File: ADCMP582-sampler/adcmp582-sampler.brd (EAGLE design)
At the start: 160 x 100 mm, 62 parts, among them IC12 MC79M05, IC13 MC78M05, IC2 MC100EPT21, IC3 SY89296U, IC6 AD711

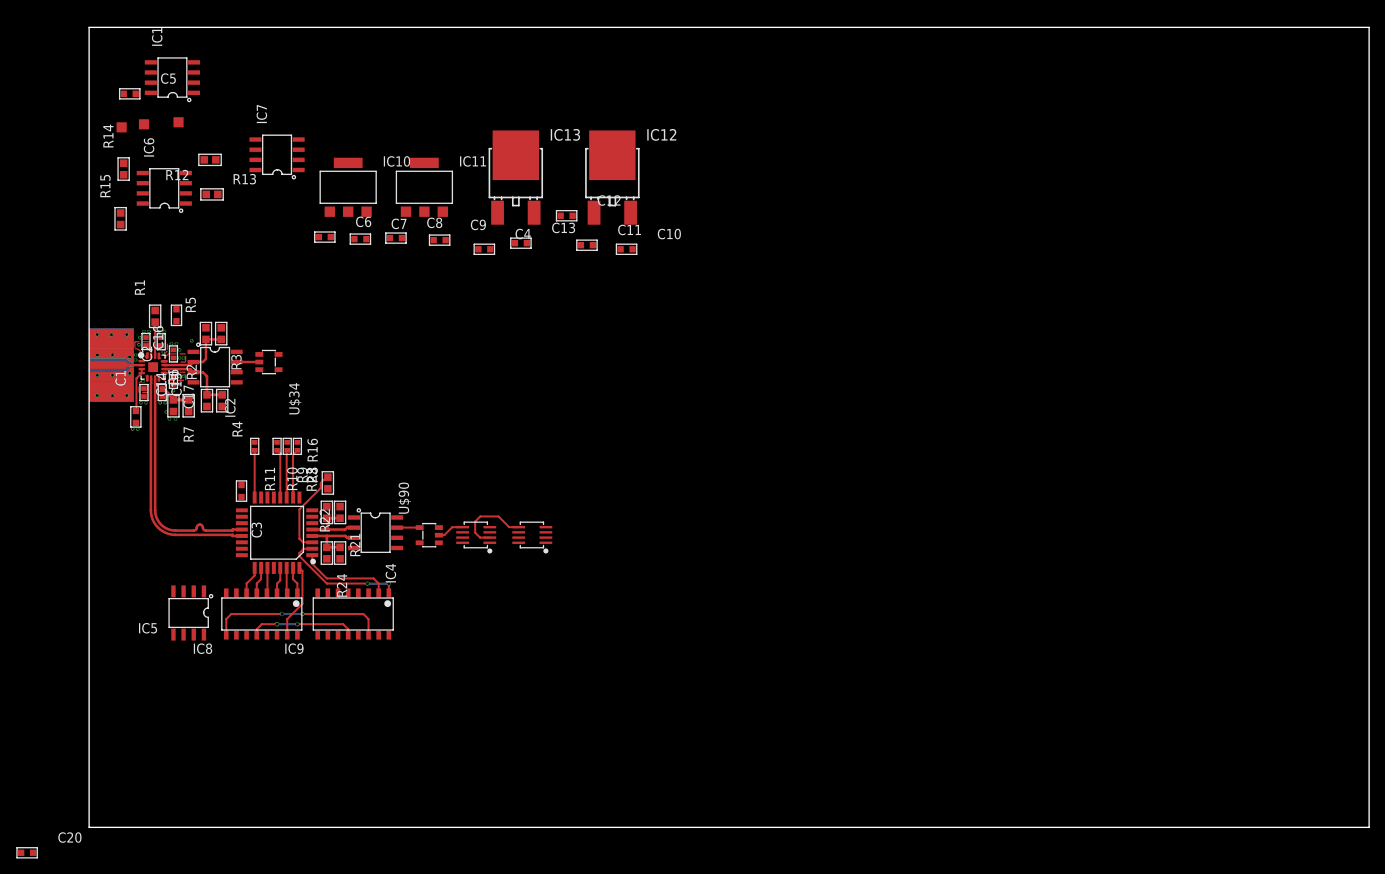
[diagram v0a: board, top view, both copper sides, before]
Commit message: checkpoint
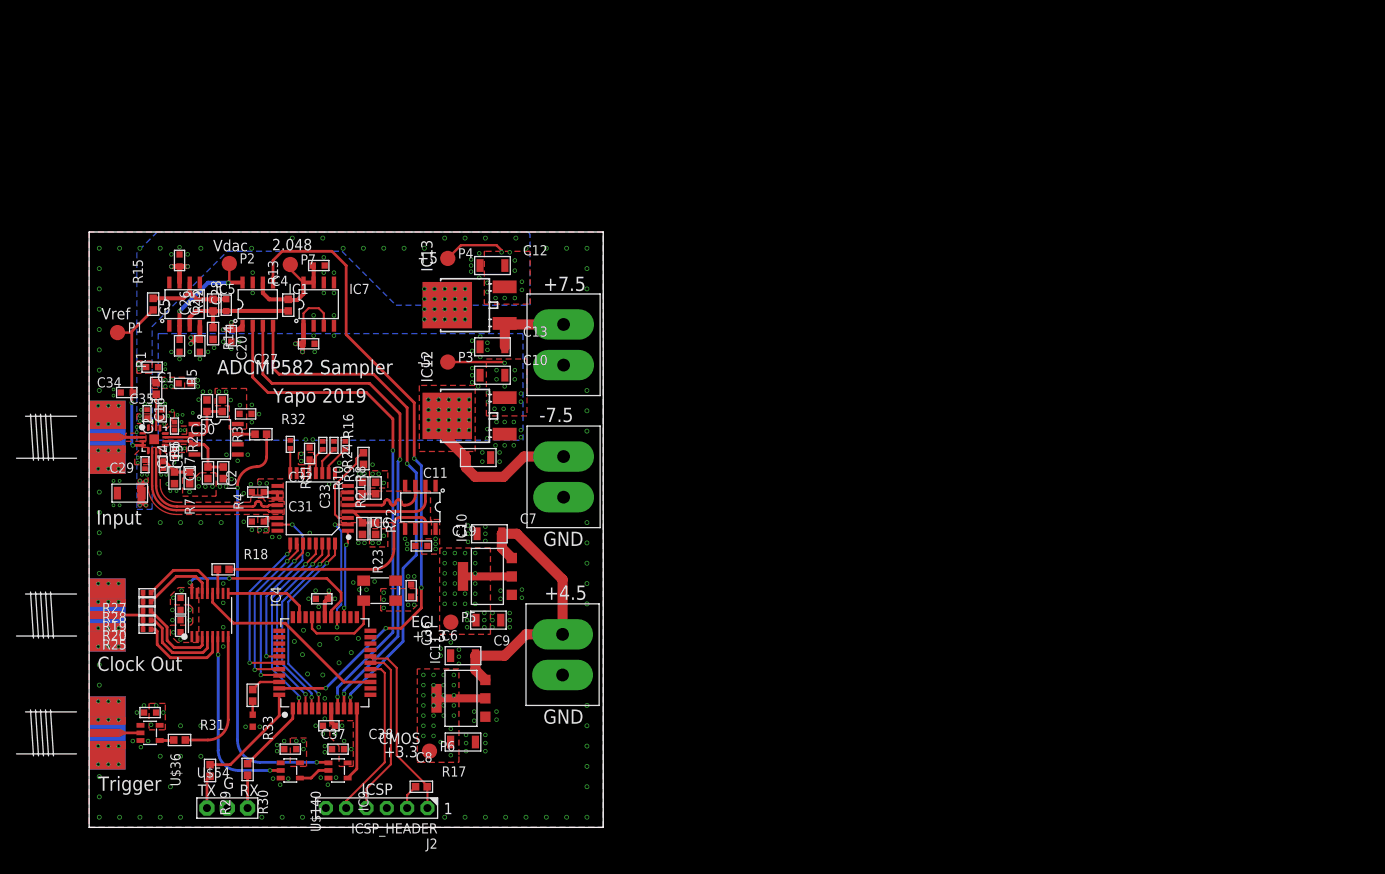
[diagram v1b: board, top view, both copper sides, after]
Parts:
- removed IC14, IC15: (no value), yapo:SSOP8
- removed U$34, U$90: 74LVC1G04, yapo:SOT23-5
- removed U$46, U$47, U$48: PAD50MIL, yapo:PAD_50MIL
- added C21, C22, C23, C24, C25, C26, C27, C28, C30, C31, C32, C33, C34, C35, C36, C37, C38: (no value), yapo:C0603
- added C29: (no value), yapo:1206
- added J2: ICSP_HEADER, yapo:HEADER_6PIN
- added J3, J4: (no value), sma_footprint_2l:SMA_EDGE_LAUNCH_4L_4020_TAPER_FIXED
- added J5, J6, J7: (no value), yapo:FCI_20020316_SCREW_TERM_2P
- added P1, P2, P3, P4, P5, P6, P7: ICSP_PAD, yapo:ICSP_PAD
- added R17, R18, R29, R30, R31, R32, R33: (no value), yapo:R0603
- added R19, R20, R25, R27, R28: (no value), yapo:0402
- added U$140: 74LVC1G04, yapo:SOT23-5
- added U$36: (no value), yapo:SOT23-5
- added U$54: HEADER_3PIN, yapo:HEADER_3PIN
- added U$88: LED_0603, yapo:LED_0603
- added X1: (no value), yapo:XTAL_3.2X5
- C10, C11, C12, C13, C6, C7, C8, C9: device yapo:C0603 -> yapo:1206
- IC4: device yapo:SOIC8 -> yapo:TQFP44
- IC6: value AD711 -> (none)
- IC8: device yapo:SOIC-16 -> yapo:TSSOP16
- IC9: device yapo:SOIC-16 -> yapo:SOT23-5
- J1: device yapo:SMA_EDGE_LAUNCH -> sma_footprint_2l:SMA_EDGE_LAUNCH_4L_4020_TAPER_FIXED
- moved C20 72.8 mm to (17.1, 65.3), turned to 270 degrees
- moved IC11 64.0 mm to (46.5, 16.1), turned to 90 degrees
- moved C8 63.5 mm to (46.7, 10.7), turned to 180 degrees
- moved C6 52.1 mm to (49.9, 25.9), turned to 180 degrees
- moved C9 52.0 mm to (46.7, 21.5)
- moved IC10 51.7 mm to (49.8, 31.4), turned to 90 degrees
- moved IC6 51.1 mm to (41.4, 40.0), turned to 180 degrees
- moved C19 42.0 mm to (41.5, 35.2), turned to 0 degrees
- moved C7 40.2 mm to (50.0, 36.7)
- moved IC5 38.6 mm to (11.9, 65.4), turned to 0 degrees
- moved C5 32.1 mm to (11.3, 60.2), turned to 90 degrees
- moved IC1 30.3 mm to (21.1, 65.4), turned to 0 degrees
- moved C11 29.8 mm to (48.6, 46.2), turned to 180 degrees
- moved IC12 28.7 mm to (51.9, 51.4), turned to 90 degrees
- moved C10 23.0 mm to (50.4, 56.5)
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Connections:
- net LE_P renamed LE_P1
- removed net N$28: C9.P$2, IC11.3
- removed net N$29: C6.P$2, IC10.2, IC10.4
- removed net N$30: C8.P$2, IC11.2, IC11.4
- removed net N$31: C11.P$2, IC12.4
- removed net N$32: C10.P$2, IC12.3
- removed net N$33: C13.P$2, IC13.1
- removed net N$34: C12.P$2, IC13.3
- removed net N$40: IC14.1, IC15.1
- removed net RCLK: IC8.12, IC9.12
- removed net SER: IC8.14
- removed net SRCLK: IC8.11, IC9.11
- removed net TUNE-!CS!: IC5.2
- removed net TUNE-SCK: IC5.3
- removed net TUNE-SDI: IC5.4
- new net !LDAC!: IC1.5, IC4.43
- new net !MCLR!: IC4.18, J2.1, R17.P$2
- new net CLK-SEL: IC4.27, IC8.16
- new net CLOCK-OUT: J4.CENTER@1, J4.P$3, R19.2, R20.2, R25.2, R27.2, R28.2
- new net COMP-CLK: IC4.14, IC8.12
- new net COMP-OUT: IC4.11, IC9.4
- new net COMP-REG-CLK: IC8.6, U$140.2
- new net ICSPCLK: IC4.16, J2.5
- new net ICSPDAT: IC4.17, J2.4
- new net INPUT: J1.CENTER@1, J1.P$3, U$1.2
- new net N$26: R33.P$2, U$88.A
- new net N$39: IC8.13, R27.1
- new net N$41: IC8.5, R25.1
- new net N$43: IC8.3, R19.1
- new net N$44: IC4.44, R29.P$1
- new net N$45: IC4.1, R30.P$1
- new net N$47: IC4.35
- new net N$48: IC4.36
- new net N$49: IC4.37
- new net N$52: IC3.17
- new net N$53: IC4.19
- new net N$54: IC4.20
- new net N$55: IC4.21
- new net N$56: IC4.22
- new net N$57: IC4.23
- new net N$58: IC4.24
- new net N$60: IC4.31
- new net RX: R30.P$2, U$54.3
- new net SAMPLE-CLOCK: IC4.32, IC8.9
- new net TRIGGER: J3.CENTER@1, J3.P$3, U$36.2
- new net TX: R29.P$2, U$54.1
- new net VCC2: C22.P$2, C23.P$2, C24.P$2, C36.P$2, C37.P$2, C38.P$2, C8.P$2, IC11.2, IC11.4, IC4.28, IC4.7, IC9.5, J2.2, P6.P$1, R17.P$1, U$140.5, U$36.5, X1.4
- new net VDAC: C5.P$2, IC1.8, IC5.2, P2.P$1
- new net VIN+5: C13.P$2, IC13.1, J6.P$1
- new net VIN-5: C11.P$2, IC12.4, J5.P$1
- new net VIN3.3: C7.P$2, C9.P$2, IC10.3, IC11.3, J7.P$1
- net +3.3V: now also C19.P$2, C21.P$2, C27.P$2, C28.P$2, C3.P$2, C30.P$2, C31.P$2, C32.P$2, C33.P$2, C6.P$2, IC10.2, IC10.4, IC6.8, IC8.1, IC8.15, IC8.2, P5.P$1; no longer IC14.6, IC14.7, IC14.8, IC15.6, IC15.7, IC15.8, IC4.8, IC5.1, IC5.6, IC8.10, IC8.16, IC9.10, IC9.16, U$34.5, U$90.5
- net +5V: now also C12.P$2, C25.P$2, C29.P$2, C34.P$2, IC13.3, IC5.7, P4.P$1; no longer IC6.7
- net -5V: now also C10.P$2, C26.P$2, C35.P$2, IC12.3, IC5.4, P3.P$1; no longer C19.P$2, IC6.4, U$48.P$1
- net D0: now also IC4.38; no longer IC8.7
- net D1: now also IC4.39; no longer IC8.6
- net D2: now also IC4.40; no longer IC8.5
- net D3: now also IC4.41; no longer IC8.4
- net D4: now also IC4.2; no longer IC8.3
- net D5: now also IC4.3; no longer IC8.2
- net D6: now also IC4.4; no longer IC8.1
- net D7: now also IC4.5; no longer IC8.15
- net D8: now also IC4.25; no longer IC9.2
- net D9: now also IC4.26; no longer IC9.1
- net GND: now also C21.P$1, C22.P$1, C23.P$1, C24.P$1, C25.P$1, C26.P$1, C27.P$1, C28.P$1, C29.P$1, C30.P$1, C31.P$1, C32.P$1, C33.P$1, C34.P$1, C35.P$1, C36.P$1, C37.P$1, C38.P$1, IC4.29, IC4.6, IC6.5, IC8.10, IC8.7, IC9.3, J1.BOTTOM_GND, J1.P$1, J1.P$2, J2.3, J3.BOTTOM_GND, J3.GND@1, J3.GND@14, J3.GND@15, J3.GND@16, J3.GND@17, J3.GND@2, J3.GND@3, J3.GND@4, J3.GND@5, J3.GND@6, J3.GND@7, J3.GND@8, J3.GND_PAD1, J3.GND_PAD2, J3.P$1, J3.P$2, J4.BOTTOM_GND, J4.GND@1, J4.GND@14, J4.GND@15, J4.GND@16, J4.GND@17, J4.GND@2, J4.GND@3, J4.GND@4, J4.GND@5, J4.GND@6, J4.GND@7, J4.GND@8, J4.GND_PAD1, J4.GND_PAD2, J4.P$1, J4.P$2, J5.P$2, J6.P$2, J7.P$2, U$140.3, U$36.3, U$54.2, U$88.C, X1.2; no longer IC1.5, IC14.4, IC15.4, IC4.5, IC5.5, IC5.7, IC8.13, IC8.8, IC9.13, IC9.8, J1.BOTTOM_PAD, U$34.3, U$90.3
- net N$1: now also R31.P$1, U$36.4; no longer J1.CENTER@1, J1.CENTER@2, U$1.2
- net N$16: now also IC3.4, IC6.2; no longer IC3.5, IC4.2
- net N$17: now also IC2.7, R32.P$1; no longer IC3.4, IC4.3, R22.P$2, R24.P$1
- net N$18: now also IC8.11, R18.P$1; no longer C3.P$2, IC3.17, IC5.8
- net N$19: now also IC9.2, U$140.4; no longer IC2.7, U$34.2
- net N$20: now also IC5.3; no longer IC6.2
- net N$21: now also IC5.6; no longer IC6.6
- net N$22: now also IC3.5, R22.P$2, R24.P$1; no longer C5.P$2, IC1.8
- net N$23: now also IC8.8, R31.P$2; no longer IC6.1, U$47.P$1
- net N$24: now also IC4.30, X1.3; no longer IC6.5, U$46.P$1
- net N$25: now also IC4.42, R33.P$1; no longer IC8.9, IC9.14
- net N$27: now also IC9.1, R32.P$2; no longer C7.P$2, IC10.3
- net N$36: now also IC6.7, R18.P$2; no longer IC4.7, U$90.4
- net N$38: now also IC8.14, R28.1; no longer IC14.5, IC15.2
- net N$42: now also IC8.4, R20.1; no longer IC15.5, U$90.2
- net V2.048: now also P7.P$1
- net VREF: now also P1.P$1
- net VREF-!CS!: now also IC4.8
- net VREF-SCK: now also IC4.9
- net VREF-SDI: now also IC4.10
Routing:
- net !LDAC!: track 0.00 -> 81.7 mm, vias 0 -> 4
- net VREF-SDI: track 0.00 -> 65.6 mm, vias 0 -> 2
- net VREF-!CS!: track 0.00 -> 65.2 mm, vias 0 -> 2
- net VREF-SCK: track 0.00 -> 65.0 mm, vias 0 -> 2
- net N$27: track 0.00 -> 52.3 mm, vias 0 -> 2
- net VIN3.3: track 0.00 -> 35.9 mm
- net N$36: track 2.81 -> 30.2 mm
- net +3.3V: track 0.00 -> 26.3 mm, vias 4 -> 63
- net COMP-CLK: track 0.00 -> 25.0 mm
- net CLK-SEL: track 0.00 -> 24.9 mm, vias 0 -> 2
- net COMP-REG-CLK: track 0.00 -> 23.1 mm, vias 0 -> 2
- net !MCLR!: track 0.00 -> 23.0 mm
- net D0: track 0.00 -> 22.4 mm, vias 0 -> 2
- net ICSPDAT: track 0.00 -> 21.5 mm
- net D5: track 3.15 -> 24.4 mm, vias 0 -> 2
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- added copper zone on layer 15, net +3.3V
- added copper zone on layer 16, net +5V
- added copper zone on layer 16, net -5V
- added copper zone on layer 1, net GND
- added copper zone on layer 16, net GND
- added copper zone on layer 2, net GND
- added copper zone on layer 1, net VCC2
- added copper zone on layer 15, net VCC2
- added copper zone on layer 1, net VIN-5
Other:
- board size 160 x 100 mm -> 64.3 x 74.4 mm
- board text added: "+3.3"
- board text added: "+4.5"
- board text added: "+5"
- board text added: "+7.5"
- board text added: "-5"
- board text added: "-7.5"
- board text added: "1"
- board text added: "2.048"
- board text added: "ADCMP582 Sampler"
- board text added: "CMOS"
- board text added: "Clock Out"
- board text added: "ECL"
- board text added: "G"
- board text added: "GND"
- board text added: "ICSP"
- board text added: "Input"
- board text added: "RX"
- board text added: "TX"
- board text added: "Trigger"
- board text added: "Vdac"
- board text added: "Vref"
- board text added: "Yapo 2019"

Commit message: checkpoint
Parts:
- R12: value (none) -> 20k
- R13, R14: value (none) -> 10k
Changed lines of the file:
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@@
 <attribute name="VALUE" x="23.876" y="45.339" size="1.27" layer="27" rot="R270"/>
 </element>
-<element name="R12" library="yapo" package="R0603" value="" x="15.494" y="61.722" smashed="yes" rot="R90">
+<element name="R12" library="yapo" package="R0603" value="20k" x="15.494" y="61.722" smashed="yes" rot="R90">
 <attribute name="NAME" x="14.224" y="64.262" size="1.27" layer="25" rot="R90"/>
 <attribute name="VALUE" x="16.764" y="64.262" size="1.27" layer="27" rot="R90"/>
 </element>
-<element name="R13" library="yapo" package="R0603" value="" x="24.892" y="65.278" smashed="yes" rot="R90">
+<element name="R13" library="yapo" package="R0603" value="10k" x="24.892" y="65.278" smashed="yes" rot="R90">
 <attribute name="NAME" x="23.622" y="67.818" size="1.27" layer="25" rot="R90"/>
 <attribute name="VALUE" x="26.162" y="67.818" size="1.27" layer="27" rot="R90"/>
 </element>
-<element name="R14" library="yapo" package="R0603" value="" x="15.494" y="65.278" smashed="yes" rot="R270">
+<element name="R14" library="yapo" package="R0603" value="10k" x="15.494" y="65.278" smashed="yes" rot="R270">
 <attribute name="NAME" x="16.764" y="62.738" size="1.27" layer="25" rot="R270"/>
 <attribute name="VALUE" x="14.224" y="62.738" size="1.27" layer="27" rot="R270"/>
@@
 <contactref element="U$140" pad="2"/>
 <via x="16.129" y="21.59" extent="1-16" drill="0.35"/>
-<wire x1="16.129" y1="21.59" x2="16.129" y2="9.652" width="0.34925" layer="16"/>
+<wire x1="16.129" y1="9.652" x2="16.129" y2="21.59" width="0.34925" layer="16"/>
 <wire x1="16.129" y1="9.652" x2="18.669" y2="7.112" width="0.34925" layer="16" curve="90"/>
 <wire x1="18.669" y1="7.112" x2="22.606" y2="7.112" width="0.34925" layer="16"/>

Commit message: checkpoint
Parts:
- C1, C20, C4, C5, R15: value (none) -> 0
- IC1: value (none) -> MCP4921
- IC10, IC11: value (none) -> AZ1117E
- IC4: value (none) -> PIC16F15376
- IC5: value (none) -> ADA4000
- IC6: value (none) -> MC100LVELT20
- IC7: value (none) -> MCP1501
- IC8: value (none) -> SI53360
- IC9: value (none) -> 74LVC1G79
- U$36: value (none) -> 74LVC1G17
- X1: value (none) -> XTAL-3.2X5-8MHz
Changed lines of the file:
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@@
 </autorouter>
 <elements>
-<element name="C1" library="yapo" package="C0603" value="" x="4.699" y="54.356" smashed="yes">
+<element name="C1" library="yapo" package="C0603" value="0" x="4.699" y="54.356" smashed="yes">
 <attribute name="NAME" x="8.509" y="55.626" size="1.27" layer="25"/>
 <attribute name="VALUE" x="8.509" y="53.086" size="1.27" layer="27"/>
@@
 <attribute name="VALUE" x="10.541" y="49.149" size="1.27" layer="27" rot="R90"/>
 </element>
-<element name="C4" library="yapo" package="C0603" value="" x="28.702" y="70.231" smashed="yes" rot="R180">
+<element name="C4" library="yapo" package="C0603" value="0" x="28.702" y="70.231" smashed="yes" rot="R180">
 <attribute name="NAME" x="24.892" y="68.961" size="1.27" layer="25" rot="R180"/>
 <attribute name="VALUE" x="24.892" y="71.501" size="1.27" layer="27" rot="R180"/>
 </element>
-<element name="C5" library="yapo" package="C0603" value="" x="11.303" y="60.198" smashed="yes" rot="R90">
+<element name="C5" library="yapo" package="C0603" value="0" x="11.303" y="60.198" smashed="yes" rot="R90">
 <attribute name="NAME" x="10.033" y="64.008" size="1.27" layer="25" rot="R90"/>
 <attribute name="VALUE" x="12.573" y="64.008" size="1.27" layer="27" rot="R90"/>
@@
 <attribute name="VALUE" x="50.546" y="20.193" size="1.27" layer="27"/>
 </element>
-<element name="IC1" library="yapo" package="SOIC8" value="" x="21.082" y="65.405" smashed="yes">
+<element name="IC1" library="yapo" package="SOIC8" value="MCP4921" x="21.082" y="65.405" smashed="yes">
 <attribute name="NAME" x="24.892" y="66.675" size="1.27" layer="25"/>
 <attribute name="VALUE" x="24.892" y="64.135" size="1.27" layer="27"/>
 </element>
-<element name="IC10" library="yapo" package="SOT-223" value="" x="49.784" y="31.369" smashed="yes" rot="R90">
+<element name="IC10" library="yapo" package="SOT-223" value="AZ1117E" x="49.784" y="31.369" smashed="yes" rot="R90">
 <attribute name="NAME" x="47.184" y="35.669" size="1.27" layer="25" rot="R90"/>
 <attribute name="VALUE" x="48.984" y="35.669" size="1.27" layer="27" rot="R90"/>
 </element>
-<element name="IC11" library="yapo" package="SOT-223" value="" x="46.482" y="16.129" smashed="yes" rot="R90">
+<element name="IC11" library="yapo" package="SOT-223" value="AZ1117E" x="46.482" y="16.129" smashed="yes" rot="R90">
 <attribute name="NAME" x="43.882" y="20.429" size="1.27" layer="25" rot="R90"/>
 <attribute name="VALUE" x="45.682" y="20.429" size="1.27" layer="27" rot="R90"/>
@@
 </element>
 <element name="IC3" library="yapo" package="TQFP32_7X7" value="SY89296U" x="27.94" y="39.878" smashed="yes" rot="R180"/>
-<element name="IC7" library="yapo" package="SOIC8" value="" x="28.702" y="65.405" smashed="yes">
+<element name="IC7" library="yapo" package="SOIC8" value="MCP1501" x="28.702" y="65.405" smashed="yes">
 <attribute name="NAME" x="32.512" y="66.675" size="1.27" layer="25"/>
 <attribute name="VALUE" x="32.512" y="64.135" size="1.27" layer="27"/>
@@
 <attribute name="VALUE" x="14.224" y="62.738" size="1.27" layer="27" rot="R270"/>
 </element>
-<element name="R15" library="yapo" package="R0603" value="" x="8.001" y="65.405" smashed="yes" rot="R90">
+<element name="R15" library="yapo" package="R0603" value="0" x="8.001" y="65.405" smashed="yes" rot="R90">
 <attribute name="NAME" x="6.731" y="67.945" size="1.27" layer="25" rot="R90"/>
 <attribute name="VALUE" x="9.271" y="67.945" size="1.27" layer="27" rot="R90"/>
@@
 </element>
 <element name="C18" library="yapo" package="C0402_NO_THERMALS" value="" x="6.985" y="45.339" smashed="yes" rot="R90"/>
-<element name="C20" library="yapo" package="C0603" value="" x="17.145" y="65.278" smashed="yes" rot="R270">
+<element name="C20" library="yapo" package="C0603" value="0" x="17.145" y="65.278" smashed="yes" rot="R270">
 <attribute name="NAME" x="18.415" y="61.468" size="1.27" layer="25" rot="R270"/>
 <attribute name="VALUE" x="15.875" y="61.468" size="1.27" layer="27" rot="R270"/>
 </element>
-<element name="IC4" library="yapo" package="TQFP44" value="" x="29.464" y="20.574" smashed="yes" rot="R90">
+<element name="IC4" library="yapo" package="TQFP44" value="PIC16F15376" x="29.464" y="20.574" smashed="yes" rot="R90">
 <attribute name="NAME" x="23.964" y="27.574" size="1.27" layer="25" rot="R90"/>
 <attribute name="VALUE" x="25.464" y="27.574" size="1.27" layer="27" rot="R90"/>
@@
 <attribute name="VALUE" x="44.069" y="3.81" size="1.27" layer="27"/>
 </element>
-<element name="IC5" library="yapo" package="SOIC8" value="" x="11.938" y="65.405" smashed="yes">
+<element name="IC5" library="yapo" package="SOIC8" value="ADA4000" x="11.938" y="65.405" smashed="yes">
 <attribute name="NAME" x="15.748" y="66.675" size="1.27" layer="25"/>
 <attribute name="VALUE" x="15.748" y="64.135" size="1.27" layer="27"/>
 </element>
-<element name="IC6" library="yapo" package="SOIC8" value="" x="41.402" y="40.005" smashed="yes" rot="R180">
+<element name="IC6" library="yapo" package="SOIC8" value="MC100LVELT20" x="41.402" y="40.005" smashed="yes" rot="R180">
 <attribute name="NAME" x="37.592" y="38.735" size="1.27" layer="25" rot="R180"/>
 <attribute name="VALUE" x="37.592" y="41.275" size="1.27" layer="27" rot="R180"/>
 </element>
-<element name="U$36" library="yapo" package="SOT23-5" value="" x="7.62" y="11.811" smashed="yes" rot="R270">
+<element name="U$36" library="yapo" package="SOT23-5" value="74LVC1G17" x="7.62" y="11.811" smashed="yes" rot="R270">
 <attribute name="NAME" x="10.16" y="9.271" size="1.27" layer="25" rot="R270"/>
 <attribute name="VALUE" x="8.89" y="9.271" size="1.27" layer="27" rot="R270"/>
 </element>
 <element name="J3" library="sma_footprint_2l" package="SMA_EDGE_LAUNCH_4L_4020_TAPER_FIXED" value="" x="0" y="11.811" smashed="yes"/>
-<element name="IC8" library="yapo" package="TSSOP16" value="" x="15.113" y="26.543" smashed="yes"/>
+<element name="IC8" library="yapo" package="TSSOP16" value="SI53360" x="15.113" y="26.543" smashed="yes"/>
 <element name="R18" library="yapo" package="R0603" value="" x="16.764" y="32.258" smashed="yes">
 <attribute name="NAME" x="19.304" y="33.528" size="1.27" layer="25"/>
@@
 <attribute name="VALUE" x="8.128" y="56.769" size="1.27" layer="27" rot="R180"/>
 </element>
-<element name="X1" library="yapo" package="XTAL_3.2X5" value="" x="36.322" y="29.591" smashed="yes" rot="R180"/>
+<element name="X1" library="yapo" package="XTAL_3.2X5" value="XTAL-3.2X5-8MHz" x="36.322" y="29.591" smashed="yes" rot="R180"/>
 <element name="C36" library="yapo" package="C0603" value="" x="40.259" y="29.591" smashed="yes" rot="R270">
 <attribute name="NAME" x="41.529" y="25.781" size="1.27" layer="25" rot="R270"/>
@@
 <attribute name="VALUE" x="26.416" y="4.572" size="1.27" layer="27" rot="R270"/>
 </element>
-<element name="IC9" library="yapo" package="SOT23-5" value="" x="31.115" y="7.112" smashed="yes" rot="R270">
+<element name="IC9" library="yapo" package="SOT23-5" value="74LVC1G79" x="31.115" y="7.112" smashed="yes" rot="R270">
 <attribute name="NAME" x="33.655" y="4.572" size="1.27" layer="25" rot="R270"/>
 <attribute name="VALUE" x="32.385" y="4.572" size="1.27" layer="27" rot="R270"/>
